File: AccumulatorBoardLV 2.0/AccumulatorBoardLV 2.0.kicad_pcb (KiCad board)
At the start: 4 copper layers, 152.4 x 50.8 mm, 66 parts, among them J1 Contactor 1, J10 To HV Board, J11 IMD Reset, J12 TS Interlock, J13 Temp Reset, J14 To ECU, J15 Charger LV, J16 Charger Interlock, J17 Lid Interlock, J18 From HV Board, J19 Chip 1, J2 Contactor 2, J20 Chip 2, J21 Chip 3, J22 Chip 4, J3 IMD LV, J4 BMS Connector 1, J5 BMS Connector 2, J6 BMS TX, J7 BMS RX, J8 Current Sensor, J9 BMS Reset, U1 DE1A1B-L2-12V, U10 MCP3008, U11 ISO1050, U12 stm_nucleo_FK303K8, U13 MCP3008, U14 MCP3008, U2 LM555N, U3 SN754410, U4 DE1A1B-L2-12V, U5 L78S05CV-DG, U6 DE1A1B-L2-12V, U7 DK1A1B-12V, U8 ADUM4154ARIZ, U9 MCP3008

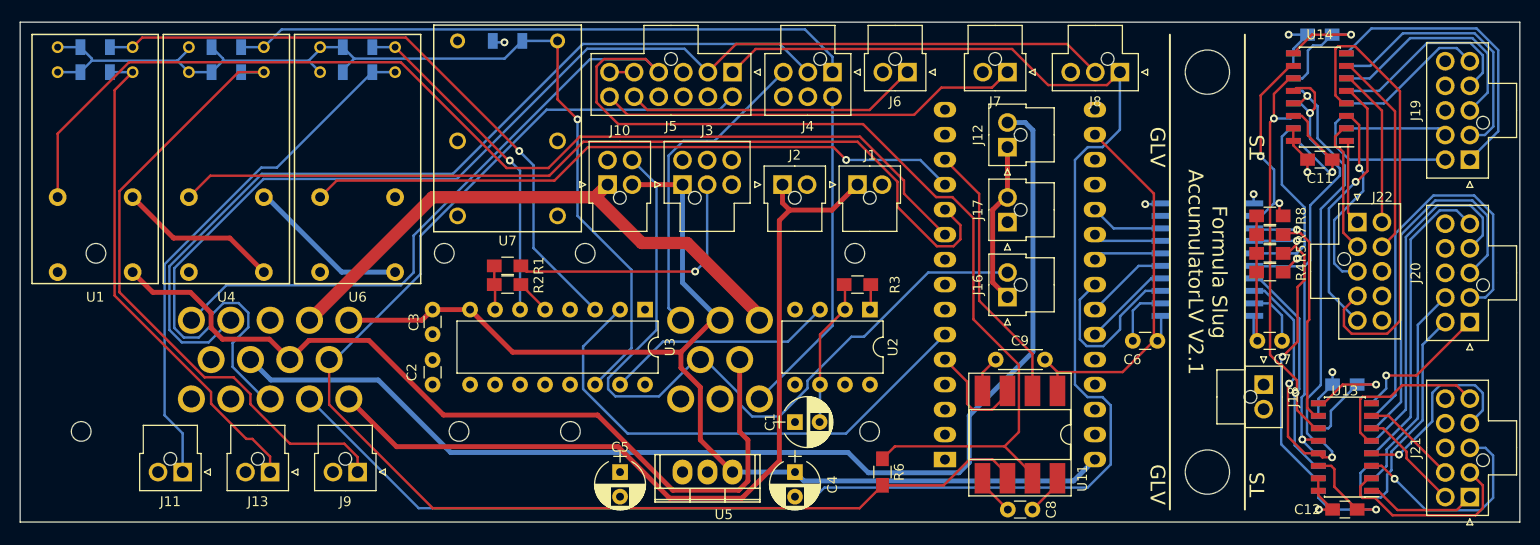
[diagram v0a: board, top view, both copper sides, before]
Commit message: final lv board routed
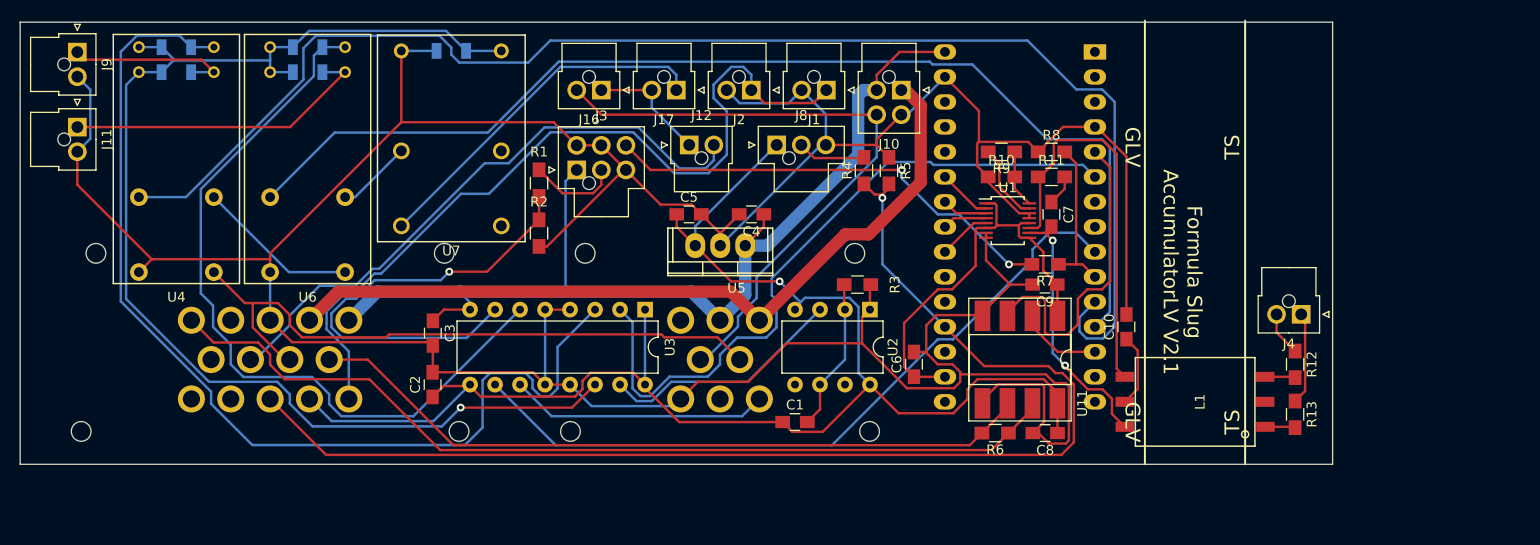
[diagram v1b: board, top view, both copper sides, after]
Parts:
- removed C11, C12, C13: 1uF, Capacitors_SMD:C_0805_HandSoldering
- removed D1, D2: D, Diodes_SMD:D_1206
- removed H1, H2: MtngHole, Mounting_Holes:MountingHole_4.5mm
- removed J13: Temp Reset, Connectors_Molex:Molex_NanoFit_1x02x2.50mm_Straight
- removed J18: From HV Board, Connectors_Molex:Molex_NanoFit_1x02x2.50mm_Straight
- removed J19: Chip 1, Connectors_Molex:Molex_NanoFit_2x05x2.50mm_Straight
- removed J20: Chip 2, Connectors_Molex:Molex_NanoFit_2x05x2.50mm_Straight
- removed J21: Chip 3, Connectors_Molex:Molex_NanoFit_2x05x2.50mm_Straight
- removed J22: Chip 4, Connectors_Molex:Molex_NanoFit_2x05x2.50mm_Straight
- removed J5: BMS Connector 2, Connectors_Molex:Molex_NanoFit_2x06x2.50mm_Straight
- removed J6: BMS TX, Connectors_Molex:Molex_NanoFit_1x02x2.50mm_Straight
- removed J7: BMS RX, Connectors_Molex:Molex_NanoFit_1x02x2.50mm_Straight
- removed U10, U13, U14, U9: MCP3008, Housings_SOIC:SOIC-16_3.9x9.9mm_Pitch1.27mm
- removed U8: ADUM4154ARIZ, Housings_SOIC:SOIC-20W_7.5x12.8mm_Pitch1.27mm
- added L1: HM2113ZNL, FSFootprints:HM2113ZNL, F.Cu at (159.7, 145.8)
- added R10: 680, Resistors_SMD:R_0805_HandSoldering, F.Cu at (140.0, 122.9)
- added R11: 402, Resistors_SMD:R_0805_HandSoldering, F.Cu at (145.1, 122.9)
- added R12: 22, Resistors_SMD:R_0805_HandSoldering, F.Cu at (169.8, 142.0)
- added R13: 22, Resistors_SMD:R_0805_HandSoldering, F.Cu at (169.8, 147.0)
- added R9: 1.5k, Resistors_SMD:R_0805_HandSoldering, F.Cu at (140.0, 120.4)
- C1, C4, C5: footprint Capacitors_THT:CP_Radial_D5.0mm_P2.50mm -> Capacitors_SMD:C_0805_HandSoldering
- C10: value 1uF -> 10nF; moved to F.Cu
- C2, C3, C6, C8: footprint Capacitors_THT:C_Disc_D3.0mm_W1.6mm_P2.50mm -> Capacitors_SMD:C_0805_HandSoldering
- C7: value 0.1uF -> 15pF; footprint Capacitors_THT:C_Disc_D3.0mm_W1.6mm_P2.50mm -> Capacitors_SMD:C_0805_HandSoldering
- C9: footprint Capacitors_THT:C_Disc_D4.3mm_W1.9mm_P5.00mm -> Capacitors_SMD:C_0805_HandSoldering
- J14: value To ECU -> To ECU in PE Box
- J4: value BMS Connector 1 -> Conn_01x02_Male; footprint Connectors_Molex:Molex_NanoFit_2x03x2.50mm_Straight -> Connectors_Molex:Molex_NanoFit_1x02x2.50mm_Straight
- R1, R2: value 1.1kR -> 1.1k
- R4, R8: value R -> 1.1k
- R5, R7: value R -> 2.2k
- U1: value DE1A1B-L2-12V -> LTC6820; footprint FSFootprints:DE1A1B-L2-12V -> FSFootprints:MSOP-16_[LTC6820]_10_thou_compat
- moved U1 96.6 mm to (140.6, 127.4)
- moved J4 53.6 mm to (170.4, 136.9)
- moved J9 51.3 mm to (46.1, 110.2), turned to 270 degrees
- moved J16 46.3 mm to (99.3, 114.1), turned to 180 degrees
- moved R4 42.5 mm to (126.0, 122.3), turned to 90 degrees
- moved R5 39.6 mm to (128.5, 122.3), turned to 270 degrees
- moved J11 36.7 mm to (46.1, 117.9), turned to 270 degrees
- moved J17 36.2 mm to (106.9, 114.1), turned to 180 degrees
- moved J8 35.7 mm to (117.1, 119.7), turned to 0 degrees
- moved C10 35.6 mm to (152.7, 138.2), turned to 90 degrees
- moved J12 32.3 mm to (108.2, 119.7), turned to 0 degrees
- moved J10 31.4 mm to (129.8, 114.1), turned to 180 degrees
- moved C5 27.1 mm to (108.2, 126.7), turned to 0 degrees
- moved C4 26.6 mm to (114.6, 126.7), turned to 180 degrees
- moved C6 24.9 mm to (131.1, 142.0), turned to 90 degrees
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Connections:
- net /12V_SRC renamed 12V_SRC
- net /AIRS_ACC_OUT renamed AIRS_ACC_OUT
- net /AIRS_FINAL renamed AIRS_FINAL
- net /AIRS_FINAL_CHARGER renamed AIRS_FINAL_CHARGER
- net /AIRS_LID_OUT renamed AIRS_LID_OUT
- net /BMS_FLT_LATCHED renamed BMS_FLT_LAT
- net /BMS_RESET renamed BMS_RESET
- net /CAN_H renamed CAN_H
- net /CAN_L renamed CAN_L
- net /CAN_RX renamed CAN_RX
- net /CAN_TX renamed CAN_TX
- net /IMD_FLT renamed IMD_FLT
- net /IMD_FLT_H renamed IMD_FLT_H
- net /IMD_FLT_LATCHED renamed IMD_FLT_LAT
- net /IMD_RESET renamed IMD_RESET
- net /TEMP_FLT renamed BMS_FLT
- net /TIMER renamed TIMER
- C10 pad 1: /3.3V_TS -> Net-(C10-Pad1)
- C10 pad 2: /BATT- -> GND
- C7 pad 1: /3.3V_TS -> Net-(C7-Pad1)
- C7 pad 2: /BATT- -> Net-(C7-Pad2)
- D3 pad 1: /TIMER_H -> TIMER_H
- D3 pad 2: /BMS_FLT -> BMS_FLT_H
- D4 pad 1: /TIMER_H -> TIMER_H
- D5 pad 1: /TIMER_H -> TIMER_H
- D6 pad 1: /TIMER_H -> TIMER_H
- D7 pad 1: /TIMER_H -> TIMER_H
- J14 pad 11: /5V_BMS -> +5V
- J14 pad 12: /SIG_CURRENT -> SIG_CURRENT
- J14 pad 4: /V_L -> (no net)
- J14 pad 7: /AIRS_CHARGER_OUT -> AIRS_CHARGER_OUT
- J15 pad 3: /V_S -> (no net)
- J15 pad 4: /AIRS_CHARGER_OUT -> AIRS_CHARGER_OUT
- J15 pad 6: /CHARGER_CONTROL -> CHARGER_CONTROL_H
- J17 pad 1: (no net) -> /AIRS_RELAYS_OUT
- J3 pad 6: (no net) -> Net-(J3-Pad6)
- J4 pad 1: /BMS_FLT -> Net-(J4-Pad1)
- J4 pad 2: /V_L -> Net-(J4-Pad2)
- J8 pad 1: /5V_BMS -> +5V
- J8 pad 2: /SIG_CURRENT -> Net-(J8-Pad2)
- R1 pad 1: /IMD_FLT_5 -> Net-(R1-Pad1)
- R2 pad 1: /IMD_FLT_5 -> GND
- R2 pad 2: GND -> Net-(R1-Pad1)
- R4 pad 1: /3.3V_TS -> SIG_CURRENT
- R4 pad 2: /TEMP_SS_0 -> Net-(J8-Pad2)
- R5 pad 1: /3.3V_TS -> GND
- R5 pad 2: /TEMP_SS_1 -> SIG_CURRENT
- R7 pad 1: /3.3V_TS -> IMD_STATUS
- R7 pad 2: /TEMP_SS_2 -> Net-(J3-Pad6)
- R8 pad 1: /3.3V_TS -> GND
- R8 pad 2: /TEMP_SS_3 -> IMD_STATUS
- U1 pad 1: /TIMER_H -> +3V3
- U1 pad 2: /TIMER_H -> Net-(U1-Pad2)
- U1 pad 3: /TEMP_FLT_LATCHED -> Net-(U1-Pad3)
- U1 pad 4: GND -> Net-(U1-Pad4)
- U1 pad 5: /AIRS_CHARGER_OUT -> Net-(U1-Pad5)
- U1 pad 6: /AIRS_TEMP_OUT -> +3V3
- U1 pad 7: /TEMP_RESET -> GND
- U1 pad 8: /TEMP_FLT_H -> GND
- U12 pad 10: /TEMP_FLT_LATCHED -> IMD_STATUS
- U12 pad 19: (no net) -> SIG_CURRENT
- U12 pad 20: Net-(U12-Pad20) -> (no net)
- U12 pad 21: Net-(U12-Pad21) -> (no net)
- U12 pad 22: Net-(U12-Pad22) -> Net-(U1-Pad5)
- U12 pad 23: Net-(U12-Pad23) -> Net-(U1-Pad4)
- U12 pad 24: Net-(U12-Pad24) -> Net-(U1-Pad3)
- U12 pad 25: Net-(U12-Pad25) -> Net-(U1-Pad2)
- U12 pad 9: (no net) -> CHARGER_CONTROL
- U3 pad 10: (no net) -> CHARGER_CONTROL
- U3 pad 11: (no net) -> CHARGER_CONTROL_H
- U3 pad 14: /TIMER_H -> TIMER_H
- U3 pad 3: /TEMP_FLT_H -> BMS_FLT_H
- U3 pad 7: /IMD_FLT_5 -> Net-(R1-Pad1)
- U4 pad 1: /TIMER_H -> TIMER_H
- U4 pad 2: /TIMER_H -> TIMER_H
- U4 pad 5: /AIRS_TEMP_OUT -> AIRS_CHARGER_OUT
- U4 pad 8: /BMS_FLT -> BMS_FLT_H
- U6 pad 1: /TIMER_H -> TIMER_H
- U6 pad 2: /TIMER_H -> TIMER_H
- U7 pad 4: (no net) -> /AIRS_RELAYS_OUT
- U7 pad 8: /TIMER_H -> TIMER_H
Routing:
- net GND: track 23.3 -> 384.5 mm, vias 2 -> 0
- net /5V_BMS: track 175.3 -> 0.00 mm
- net +5V: track 4.23 -> 151.5 mm, vias 0 -> 1
- net /SIG_CURRENT: track 134.0 -> 0.00 mm
- net TIMER_H: track 0.00 -> 126.8 mm, vias 0 -> 1
- net SIG_CURRENT: track 0.00 -> 125.7 mm, vias 0 -> 1
- net /TEMP_FLT_LATCHED: track 110.3 -> 0.00 mm
- net /TIMER_H: track 105.1 -> 0.00 mm, vias 1 -> 0
- net BMS_FLT_H: track 0.00 -> 104.4 mm
- net /V_L: track 89.6 -> 0.00 mm
- net /AIRS_CHARGER_OUT: track 87.3 -> 0.00 mm
- net /BATT-: track 77.0 -> 0.00 mm, vias 5 -> 0
- net CHARGER_CONTROL: track 0.00 -> 73.9 mm
- net /SCLK: track 67.5 -> 0.00 mm, vias 3 -> 0
- net /TEMP_FLT_H: track 66.1 -> 0.00 mm, vias 1 -> 0
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- removed copper zone on In1.Cu, net +5V
- removed copper zone on In1.Cu, net /3.3V_TS
- removed copper zone on In2.Cu, net /BATT-
- removed copper zone on In2.Cu, net GND
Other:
- board size 152.4 x 50.8 mm -> 133.4 x 44.9 mm
- copper layers 4 -> 2
- net class HighSpeed: via_dia 100 -> 100.000003; via_drill 50 -> 50.000002
- net class Power: via_dia 100 -> 100.000003
